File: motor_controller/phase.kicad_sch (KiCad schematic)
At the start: 25 parts

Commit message: silk
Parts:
- C19: footprint Capacitor_THT:C_Disc_D3.0mm_W1.6mm_P2.50mm -> project:C_Disc_D3.0mm_W1.6mm_P2.50mm_no_silk
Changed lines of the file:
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@@
 			)
 		)
-		(property "Footprint" "Capacitor_THT:C_Disc_D3.0mm_W1.6mm_P2.50mm"
+		(property "Footprint" "project:C_Disc_D3.0mm_W1.6mm_P2.50mm_no_silk"
 			(at 26.67 63.5 0)
 			(effects

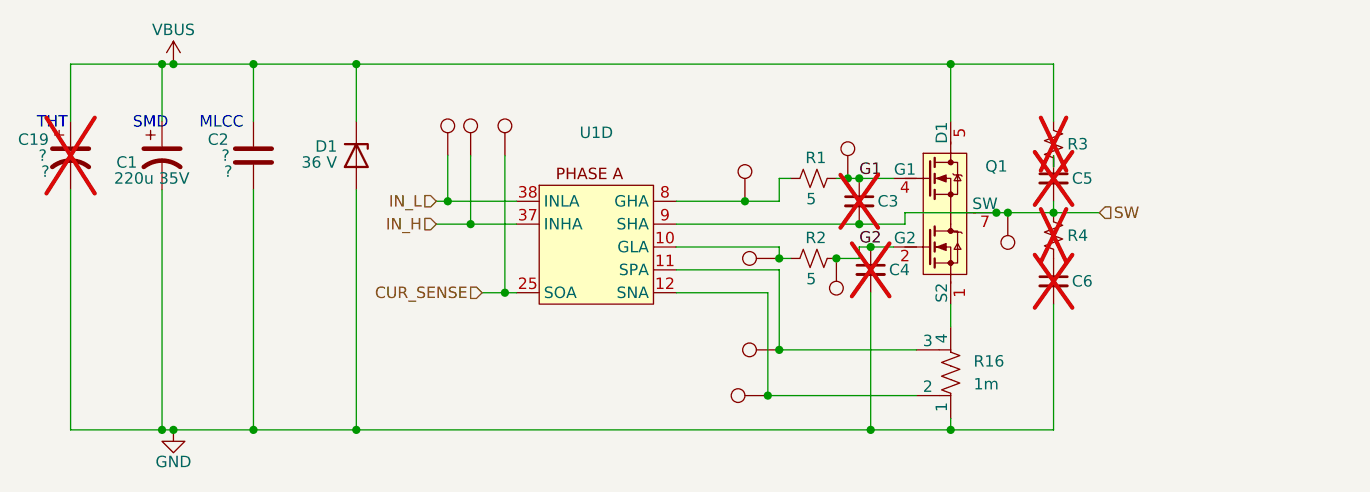
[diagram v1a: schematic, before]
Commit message: still gotta put temp sensors on lol
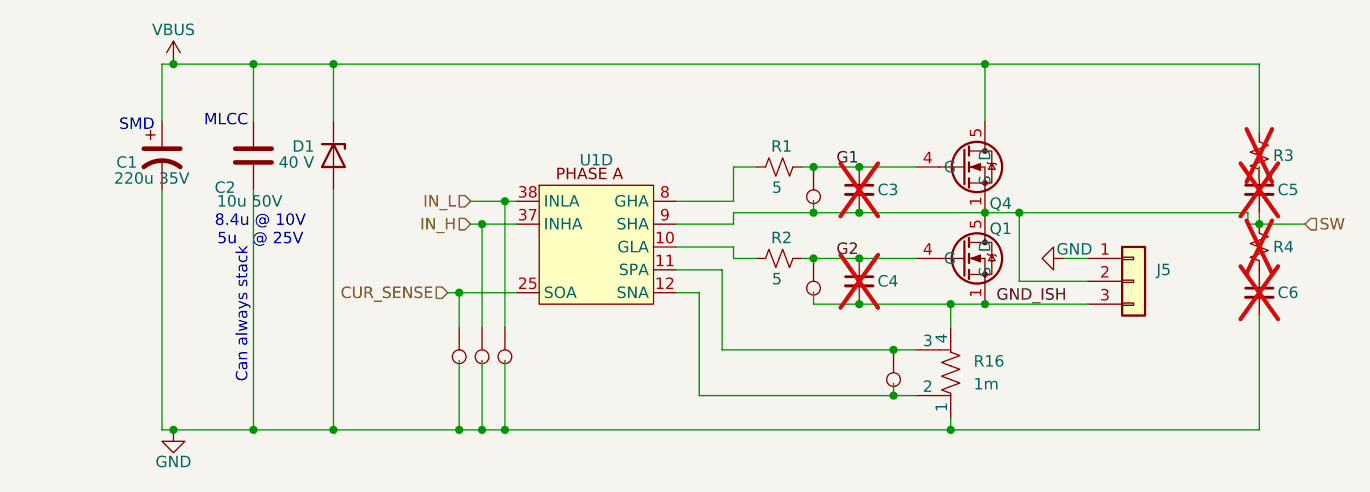
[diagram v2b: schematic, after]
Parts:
- removed C19: ?, project:C_Disc_D3.0mm_W1.6mm_P2.50mm_no_silk, symbol Device:C_Polarized_US
- removed Q1: ~, project:BUK7V4R2-40HX, symbol project:BUK7V4R2-40HX
- removed TP23, TP26, TP29, TP32, TP7: test point, project:test point d1.5, symbol project:TestPoint
- added J5: Conn_01x03, project:tp_3x, symbol Connector_Generic:Conn_01x03
- added Q1, Q4: ~, Package_SON:Infineon_PG-TDSON-8_6.15x5.15mm, symbol project:BSC110N06NS3GATMA1
- added TP7: test point, project:test point d1.5, symbol project:tp2
- C2: value ? -> 10u 50V; footprint Capacitor_SMD:C_1808_4520Metric -> Capacitor_SMD:C_1210_3225Metric; MPN ? -> CL32B106KBJNNWE; rating at vbus ? -> (none); voltage ? -> (none)
- D1: value 36 V -> 40 V; footprint Diode_SMD:D_SOD-323_HandSoldering -> Diode_SMD:D_SMA; MPN BZM55C36 -> SMAJ36A
- TP1, TP20, TP35, TP38, TP4: symbol project:TestPoint -> project:tp2
- U1: footprint (none) -> Package_DFN_QFN:VQFN-48-1EP_7x7mm_P0.5mm_EP4.1x4.1mm_ThermalVias
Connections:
- net CUR_SENSE: now also TP7.1
- net G1: now also Q4.4 (G)
- net G2: now also Q1.4 (G)
- net GND: now also TP1.2 (1), TP4.2 (1), J5.1 (Pin_1), TP7.2 (1); no longer C4.2
- net IN_H: now also TP1.1; no longer TP4.1
- net IN_L: now also TP4.1; no longer TP1.1
- net SW: now also TP35.2 (1), J5.2 (Pin_2), Q1.5 (D), Q4.1 (S), Q4.2 (S), Q4.3 (S)
- net VBUS: now also Q4.5 (D)
- net at R16.2, U1.12 (SNA): now also TP20.2 (1); no longer TP20.1
- net at R16.3, U1.11 (SPA): now also TP20.1
- net GND_ISH: now reaches R16.4
- net GND_ISH: now also C4.2, TP38.2 (1), J5.3 (Pin_3), Q1.1 (S), Q1.2 (S), Q1.3 (S)
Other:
- note added: "8.4u @ 10V 5u @ 25V"
- note added: "Can always stack"
- note removed: "THT"
- moved on the sheet: C3, C4, C5, C6, D1, R1, R2, R3, R4
